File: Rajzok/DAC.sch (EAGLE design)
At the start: 17 parts, among them Q1 TP0602N2, Q2 TP0602N2, Q3 SUP75N06-08, Q4 SUP75N06-08

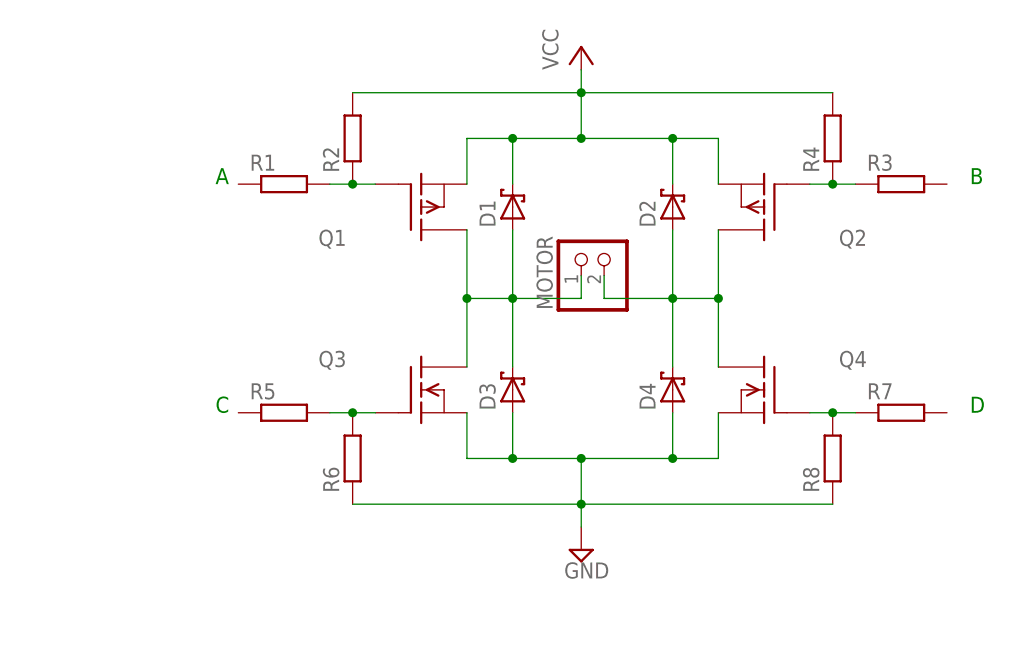
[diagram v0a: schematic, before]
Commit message: Rajzok 2017
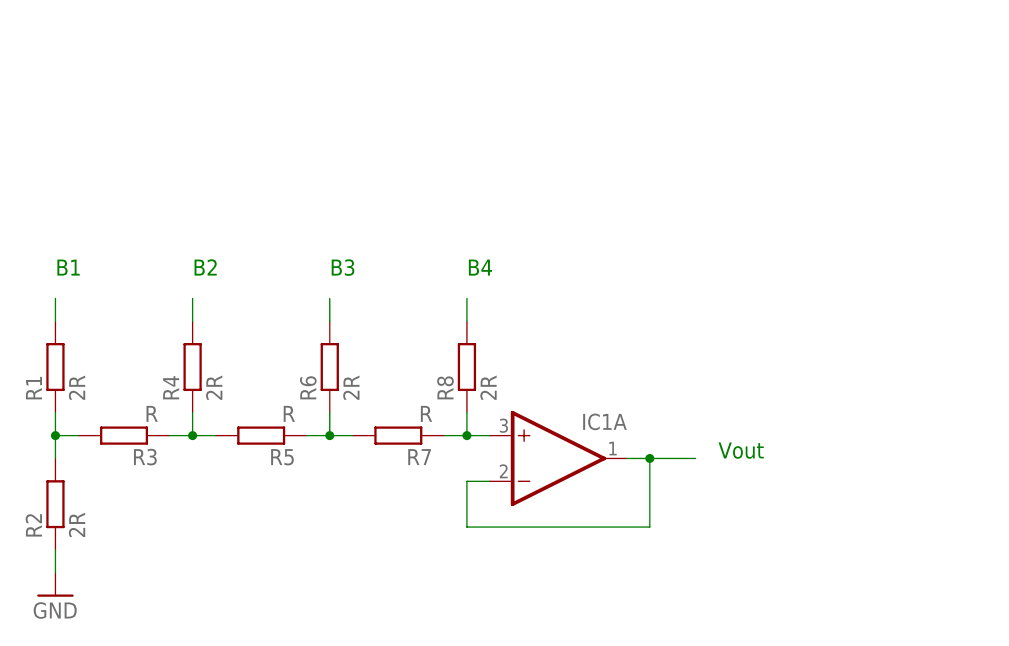
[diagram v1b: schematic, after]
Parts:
- removed D1, D2, D3, D4: 1N6267A, diode:1N6267A
- removed MOTOR: (no value), pinhead:PINHD-1X2
- removed Q1, Q2: TP0602N2, transistor-fet:TP0602N2
- removed Q3, Q4: SUP75N06-08, transistor-fet:SUP75N06-08
- added IC1: QUAD_OPAMPP, adafruit:QUAD_OPAMPP
- R1, R2, R4, R6, R8: value (none) -> 2R; device rcl:R-EU_0204/7 -> rcl:R-EU_0309/12
- R3, R5, R7: value (none) -> R; device rcl:R-EU_0204/7 -> rcl:R-EU_0309/12
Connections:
- removed net VCC: D1.C, D2.C, Q1.S, Q2.S, R2.2, R4.2
- new net N$6: R4.2
- new net N$7: R6.2
- new net N$8: R8.2
- net GND: now also R2.1; no longer D3.A, D4.A, Q3.S, Q4.S, R6.1, R8.1
- net N$1: now also R1.1, R2.2, R3.2; no longer Q1.G, R1.2, R2.1
- net N$2: now also R1.2; no longer D2.A, D4.C, MOTOR.2, Q2.D, Q4.D
- net N$3: now also R5.2; no longer Q2.G
- net N$4: now also R5.1, R6.1, R7.2; no longer Q3.G, R5.2, R6.2
- net N$5: now also IC1A.+IN, R8.1; no longer Q4.G, R8.2
- net N$9: now also IC1A.-IN, IC1A.OUT; no longer D1.A, D3.C, MOTOR.1, Q1.D, Q3.D
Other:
- note added: "B1"
- note added: "B2"
- note added: "B3"
- note added: "B4"
- note added: "Vout"
- note removed: "A"
- note removed: "B"
- note removed: "C"
- note removed: "D"
- moved on the sheet: R1, R2, R3, R4, R5, R6, R7, R8
